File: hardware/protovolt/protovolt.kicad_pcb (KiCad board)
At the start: 4 copper layers, 104.5 x 43 mm, 76 parts, among them J1 Conn_01x03, J10 Conn_02x03_Odd_Even, J2 Conn_01x03, J3 Conn_01x03, J4 Conn_01x03, J5 Conn_01x03, J6 Conn_01x03, J7 Conn_01x03, J8 Conn_01x03, J9 Conn_02x03_Odd_Even, Q1 BSC0702LS, Q2 BSC0702LS, Q3 BSC0702LS, Q4 BSC0702LS, Q5 BSC0702LS, U1 INA226, U2 LM51772RHAR

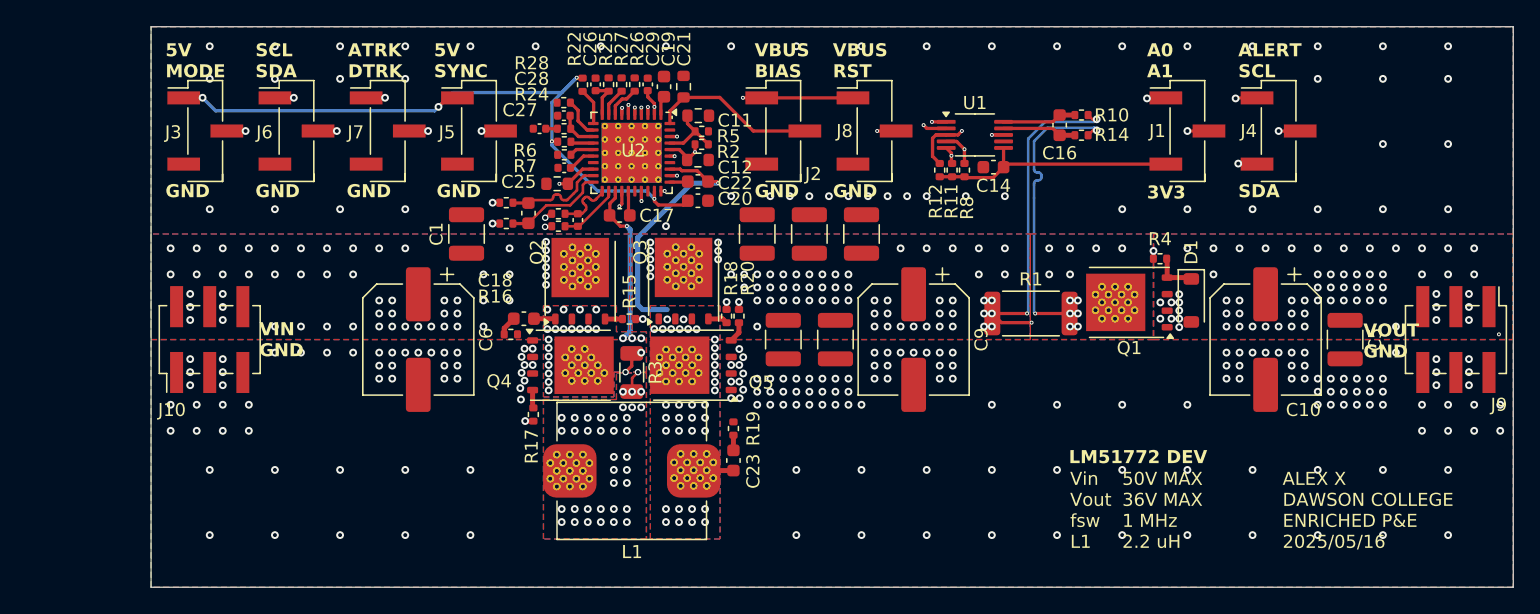
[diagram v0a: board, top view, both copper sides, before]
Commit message: replace parts
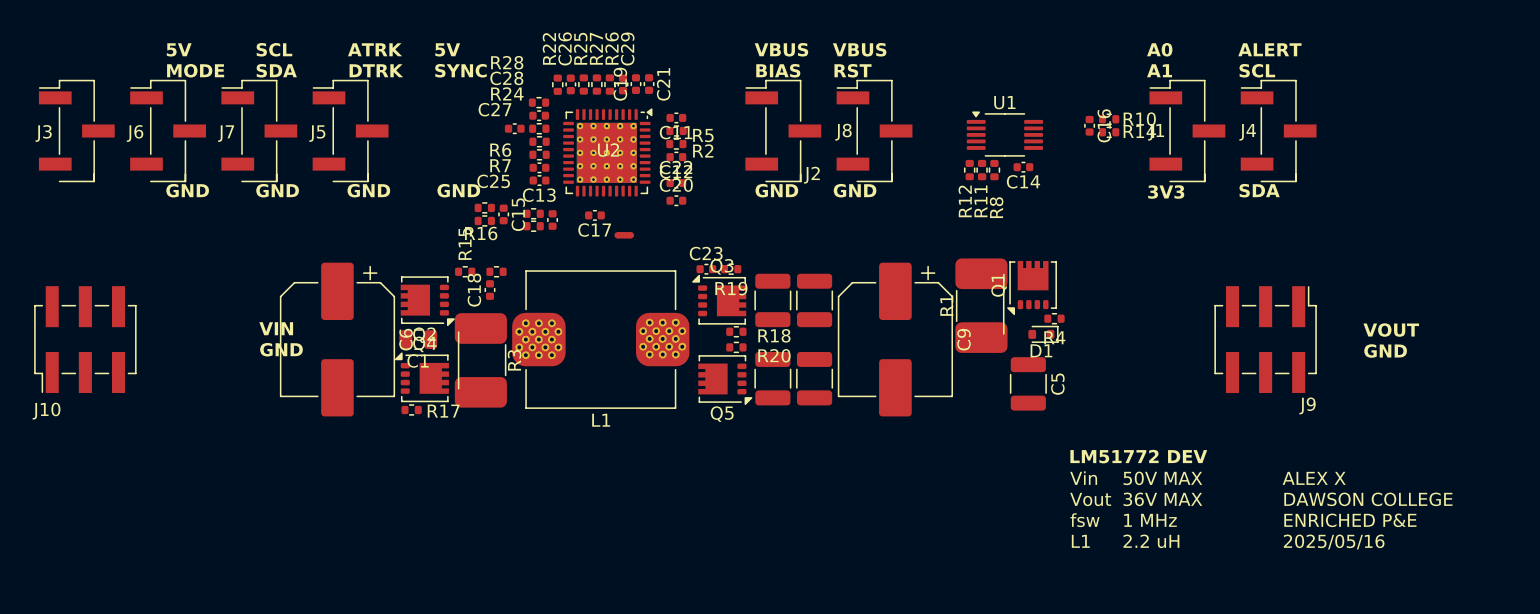
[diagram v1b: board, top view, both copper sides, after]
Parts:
- removed C10: 39u 50V, Capacitor_SMD:CP_Elec_8x11.9
- removed C4: 10u 100V, Capacitor_SMD:C_1210_3225Metric
- added NT1: NetTie_2, NetTie:NetTie-2_SMD_Pad0.5mm, F.Cu at (171.8, 112.0)
- C1: footprint Capacitor_SMD:C_1210_3225Metric -> Capacitor_SMD:C_0805_2012Metric
- C11, C12, C13, C21: footprint Resistor_SMD:R_0603_1608Metric -> Capacitor_SMD:C_0402_1005Metric
- C14, C15, C16, C17, C18, C19, C20, C22, C23: footprint Capacitor_SMD:C_0603_1608Metric -> Capacitor_SMD:C_0402_1005Metric
- C6, C9: value 39u 50V -> 47u 63V; footprint Capacitor_SMD:CP_Elec_8x11.9 -> Capacitor_SMD:CP_Elec_8x10.5
- D1: footprint Diode_SMD:D_SOD-123 -> Diode_SMD:D_SOD-523
- Q1, Q2, Q3, Q4, Q5: value BSC0702LS -> HSBB6054; footprint protovolt:TDSON-8-1 -> Package_SON:Diodes_PowerDI3333-8
- R1: footprint Resistor_SMD:R_2512_6332Metric -> protovolt:R_2512_6332Metric_SHUNT
- R3: footprint Resistor_SMD:R_1206_3216Metric -> protovolt:R_2512_6332Metric_SHUNT
- moved C5 24.5 mm to (202.8, 123.4)
- moved C23 14.8 mm to (178.1, 114.6), turned to 0 degrees
- moved J9 14.6 mm to (221.0, 120.0)
- moved R15 13.1 mm to (159.6, 114.8)
- moved R19 12.2 mm to (180.0, 114.6), turned to 0 degrees
- moved Q2 12.0 mm to (156.5, 117.0), turned to 180 degrees
- moved D1 11.8 mm to (203.8, 119.6), turned to 180 degrees
- moved R3 11.6 mm to (160.8, 121.6)
- moved Q4 11.2 mm to (156.5, 123.0)
- moved L1 10.4 mm to (170.0, 120.0)
- moved J3 9.85 mm to (129.8, 104.0)
- moved J5 9.85 mm to (150.8, 104.0)
- moved J6 9.85 mm to (136.8, 104.0)
- moved J7 9.85 mm to (143.8, 104.0)
- moved J10 9.54 mm to (130.5, 120.0)
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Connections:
- C12 pad 1: GND -> GNDA
- C13 pad 2: GND -> GNDA
- C19 pad 2: GND -> GNDA
- C21 pad 1: GND -> GNDA
- C25 pad 2: GND -> GNDA
- C26 pad 2: GND -> GNDA
- C27 pad 2: GND -> GNDA
- C28 pad 2: GND -> GNDA
- C29 pad 2: GND -> GNDA
- J2 pad 3: GND -> GNDA
- J3 pad 3: GND -> GNDA
- J5 pad 3: GND -> GNDA
- J6 pad 3: GND -> GNDA
- J7 pad 3: GND -> GNDA
- J8 pad 3: GND -> GNDA
- R25 pad 2: GND -> GNDA
- R26 pad 2: GND -> GNDA
- R27 pad 2: GND -> GNDA
- R28 pad 2: GND -> GNDA
- R7 pad 1: GND -> GNDA
- U2 pad 17: GND -> GNDA
- U2 pad 41: GND -> GNDA
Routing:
- net /output_A/ISNSR_P: track 127.1 -> 0.00 mm, vias 69 -> 0
- net /output_A/ISNSR_N: track 72.8 -> 0.00 mm, vias 15 -> 0
- net /output_A/VCC2: track 53.4 -> 0.00 mm, vias 5 -> 0
- net Net-(D1-A): track 51.8 -> 0.00 mm, vias 67 -> 0
- net VBUS: track 44.1 -> 0.00 mm, vias 57 -> 0
- net /output_A/DRV: track 41.3 -> 0.00 mm, vias 2 -> 0
- net /output_A/CSR_P: track 35.9 -> 0.00 mm, vias 25 -> 0
- net /output_A/MODE: track 34.1 -> 0.00 mm, vias 2 -> 0
- net /output_A/SCL: track 32.4 -> 0.00 mm, vias 2 -> 0
- net Net-(J4-Pin_1): track 31.8 -> 0.00 mm, vias 2 -> 0
- net Net-(J4-Pin_2): track 31.2 -> 0.00 mm, vias 2 -> 0
- net /output_A/SDA: track 28.3 -> 0.00 mm, vias 2 -> 0
- net Net-(U2-LO1): track 27.1 -> 0.00 mm, vias 2 -> 0
- net Net-(J4-Pin_3): track 27.0 -> 0.00 mm, vias 2 -> 0
- net /output_A/ATRK: track 25.4 -> 0.00 mm, vias 2 -> 0
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- removed copper zone on B.Cu, net /output_A/CSR_N
- removed copper zone on F.Cu, net /output_A/CSR_N
- removed copper zone on In1.Cu, net /output_A/CSR_N
- removed copper zone on B.Cu, net /output_A/CSR_P
- removed copper zone on F.Cu, net /output_A/CSR_P
- removed copper zone on In1.Cu, net /output_A/CSR_P
- removed copper zone on B.Cu, net /output_A/ISNSR_N
- removed copper zone on F.Cu, net /output_A/ISNSR_N
- removed copper zone on In1.Cu, net /output_A/ISNSR_N
- removed copper zone on In2.Cu, net /output_A/ISNSR_N
- removed copper zone on B.Cu, net /output_A/ISNSR_P
- removed copper zone on F.Cu, net /output_A/ISNSR_P
- removed copper zone on In1.Cu, net /output_A/ISNSR_P
- removed copper zone on In2.Cu, net /output_A/ISNSR_P
- removed copper zone on B.Cu, net /output_A/SW2
- removed copper zone on F.Cu, net /output_A/SW2
- removed copper zone on In1.Cu, net /output_A/SW2
- removed copper zone on B.Cu, net GND
- removed copper zone on F.Cu, net GND
- removed copper zone on In1.Cu, net GND
- removed copper zone on In2.Cu, net GND
- removed copper zone on B.Cu, net Net-(D1-A)
- removed copper zone on F.Cu, net Net-(D1-A)
- removed copper zone on In1.Cu, net Net-(D1-A)
- removed copper zone on In2.Cu, net Net-(D1-A)
- removed copper zone on B.Cu, net VBUS
- removed copper zone on F.Cu, net VBUS
- removed copper zone on In1.Cu, net VBUS
- removed copper zone on In2.Cu, net VBUS
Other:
- board outline removed
